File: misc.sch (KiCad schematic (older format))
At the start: 18 parts, among them J13 MICROSD_SLOT_TFP09-2-12B

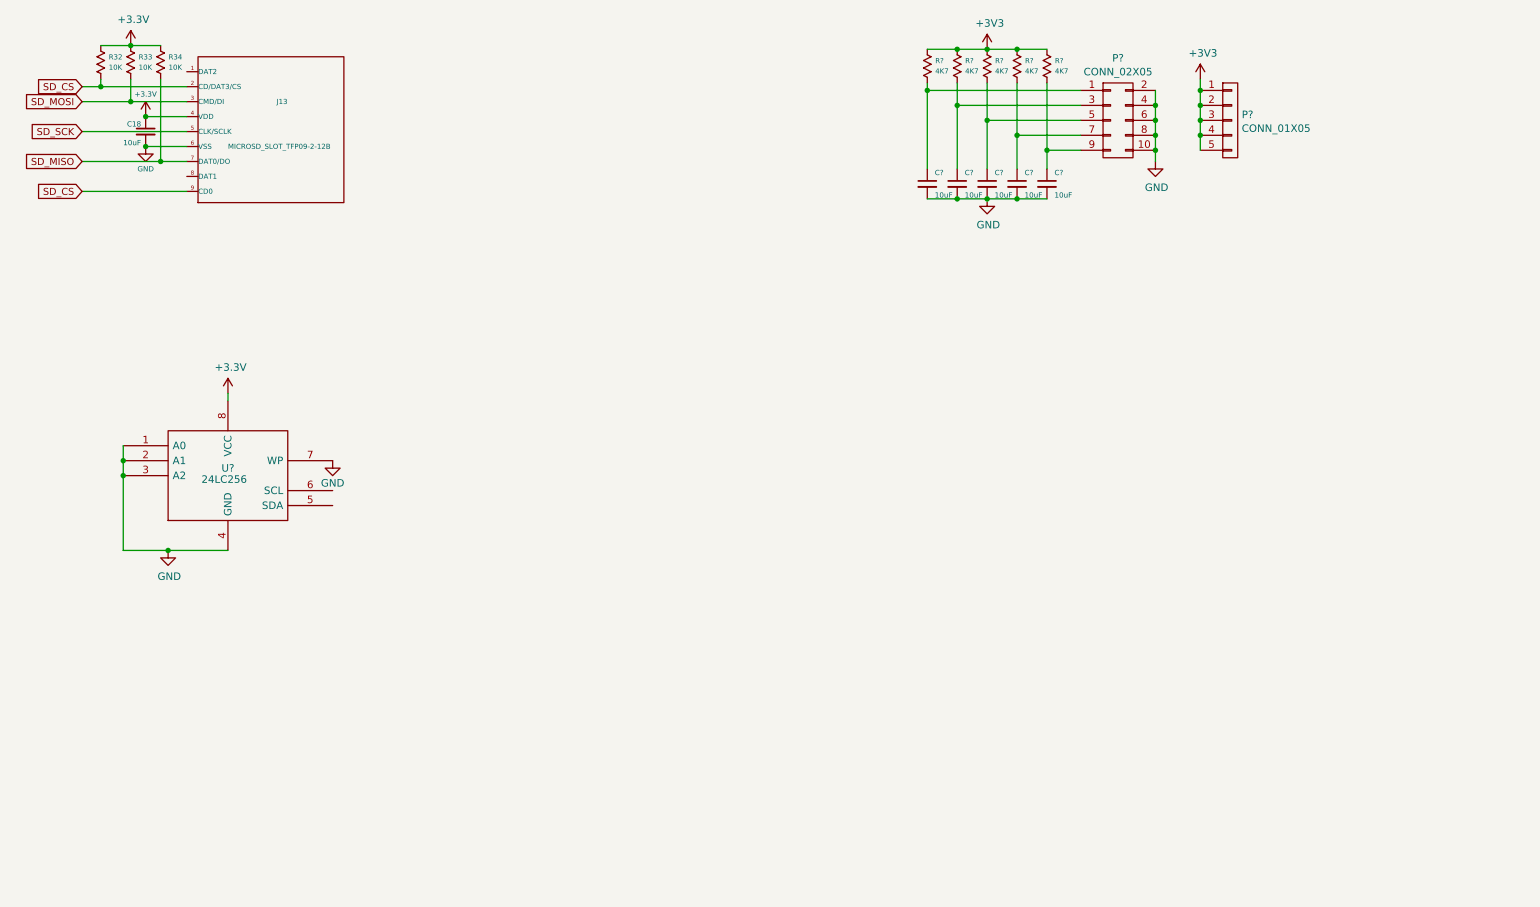
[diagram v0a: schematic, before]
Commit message: More schematics, some layout
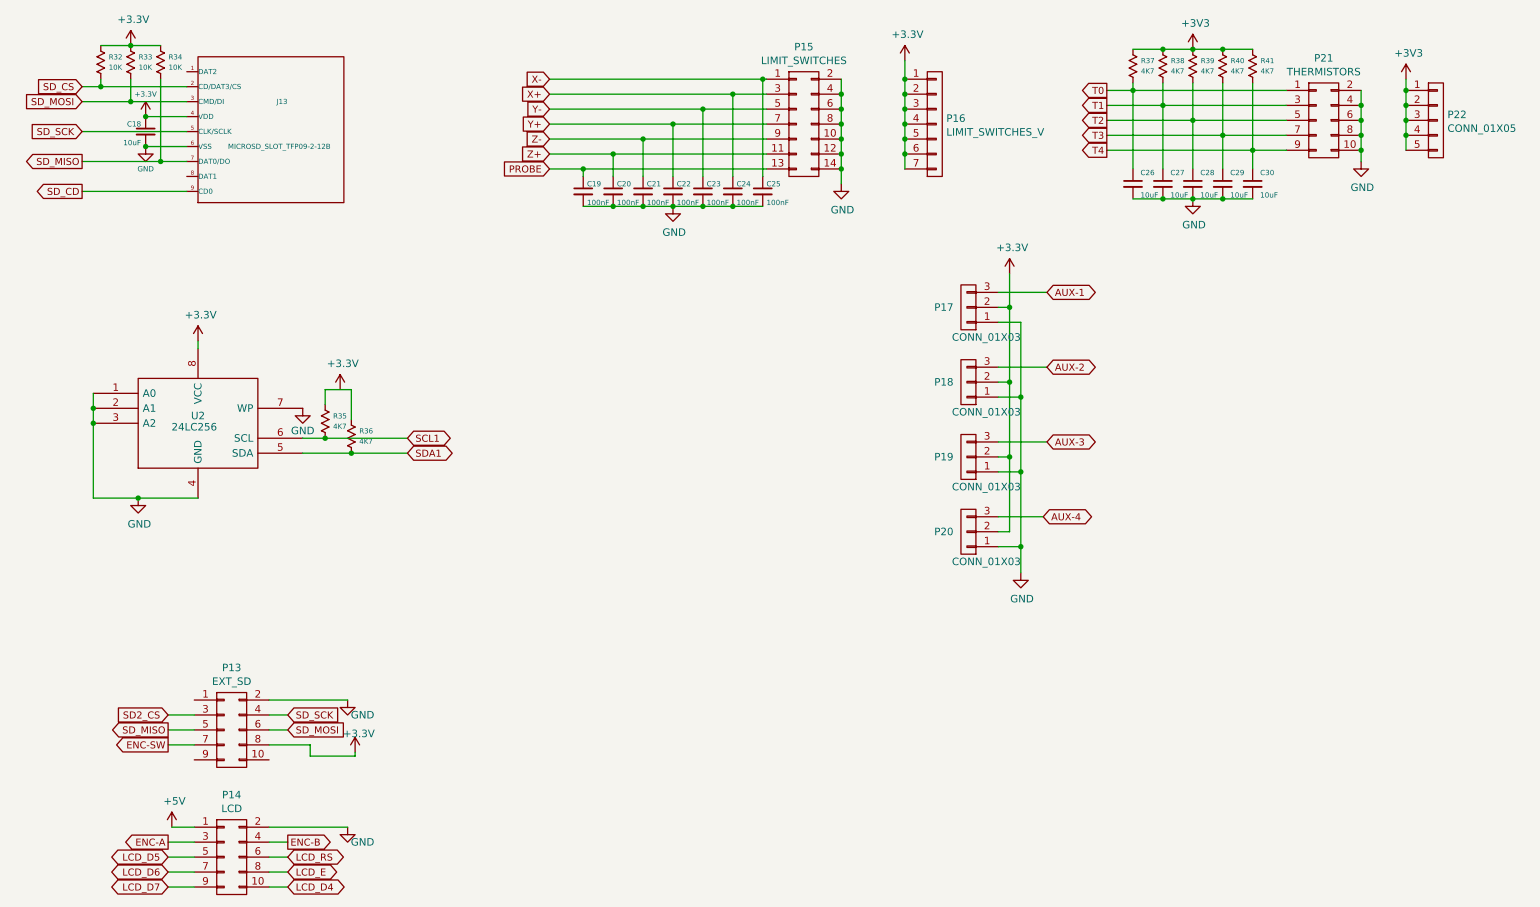
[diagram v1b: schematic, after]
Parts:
- added C19, C20, C21, C22, C23, C24, C25: 100nF, Capacitors_SMD:C_0603, symbol C_Small
- added P13: EXT_SD, geda-footprints:CON_HDR_2x5, symbol CONN_02X05
- added P14: LCD, geda-footprints:CON_HDR_2x5, symbol CONN_02X05
- added P15: LIMIT_SWITCHES, geda-footprints:CON_HDR_2x7, symbol CONN_02X07
- added P16: LIMIT_SWITCHES_V, geda-footprints:CON_HDR_1x7, symbol CONN_01X07
- added P17, P18, P19, P20: CONN_01X03, geda-footprints:CON_HDR_1x3, symbol CONN_01X03
- added R35, R36: 4K7, Resistors_SMD:R_0603, symbol RESISTOR
- C26, C27, C28, C29, C30: renamed from C?; footprint (none) -> Capacitors_SMD:C_0805
- P21: renamed from P?; value CONN_02X05 -> THERMISTORS; footprint (none) -> geda-footprints:CON_HDR_2x5
- P22: renamed from P?; footprint (none) -> geda-footprints:CON_HDR_1x5
- R37, R38, R39, R40, R41: renamed from R?; footprint (none) -> Resistors_SMD:R_0603
- U2: renamed from U?; footprint (none) -> geda-footprints:SOIC8
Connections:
- net +3V3: now also P13.8 (P8), P16.1 (P1), P16.2 (P2), P16.3 (P3), P16.4 (P4), P16.5 (P5), P16.6 (P6), P16.7 (P7), P17.2 (P2), P18.2 (P2), P19.2 (P2), P20.2 (P2)
- net GND: now also C19.2, C20.2, C21.2, C22.2, C23.2, C24.2, C25.2, P13.2 (P2), P14.2 (P2), P15.10 (P10), P15.12 (P12), P15.14 (P14), P15.2 (P2), P15.4 (P4), P15.6 (P6), P15.8 (P8), P17.1 (P1), P18.1 (P1), P19.1 (P1), P20.1 (P1)
- net SD_CS: no longer J13.9 (CD0)
- net SD_MISO: now also P13.5 (P5)
- net SD_MOSI: now also P13.6 (P6)
- net SD_SCK: now also P13.4 (P4)
- net T0: now reaches C26.1, P21.1 (P1), R37.2
- net T1: now reaches C27.1, P21.3 (P3), R38.2
- net T2: now reaches C28.1, P21.5 (P5), R39.2
- net T3: now reaches C29.1, P21.7 (P7), R40.2
- net T4: now reaches C30.1, P21.9 (P9), R41.2
- net SDA1: now reaches U2.5 (SDA)
- net SDA1: now also R36.2
- net SCL1: now reaches U2.6 (SCL)
- net SCL1: now also R35.2
- new net: R35.1, R36.1
- new net +5V: P14.1 (P1)
- new net AUX-1: P17.3 (P3)
- new net AUX-2: P18.3 (P3)
- new net AUX-3: P19.3 (P3)
- new net AUX-4: P20.3 (P3)
- new net ENC-A: P14.3 (P3)
- new net ENC-B: P14.4 (P4)
- new net ENC-SW: P13.7 (P7)
- new net LCD_D4: P14.10 (P10)
- new net LCD_D5: P14.5 (P5)
- new net LCD_D6: P14.7 (P7)
- new net LCD_D7: P14.9 (P9)
- new net LCD_E: P14.8 (P8)
- new net LCD_RS: P14.6 (P6)
- new net PROBE: C19.1, P15.13 (P13)
- new net SD2_CS: P13.3 (P3)
- new net SD_CD: J13.9 (CD0)
- new net X+: C24.1, P15.3 (P3)
- new net X-: C25.1, P15.1 (P1)
- new net Y+: C22.1, P15.7 (P7)
- new net Y-: C23.1, P15.5 (P5)
- new net Z+: C20.1, P15.11 (P11)
- new net Z-: C21.1, P15.9 (P9)
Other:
- moved on the sheet: C26, C27, C28, C29, C30, P21, P22, R37, R38, R39, R40, R41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
